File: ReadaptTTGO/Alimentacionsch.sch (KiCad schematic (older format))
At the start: 32 parts, among them J1 USB_B_Micro, J2 Conn_01x02_Shielded, SW1 SW_SPDT, U1 CP2102N-A01-GQFN24, U3 EMH3, U4 TP4054, U5 ME6211, U6 ME6211

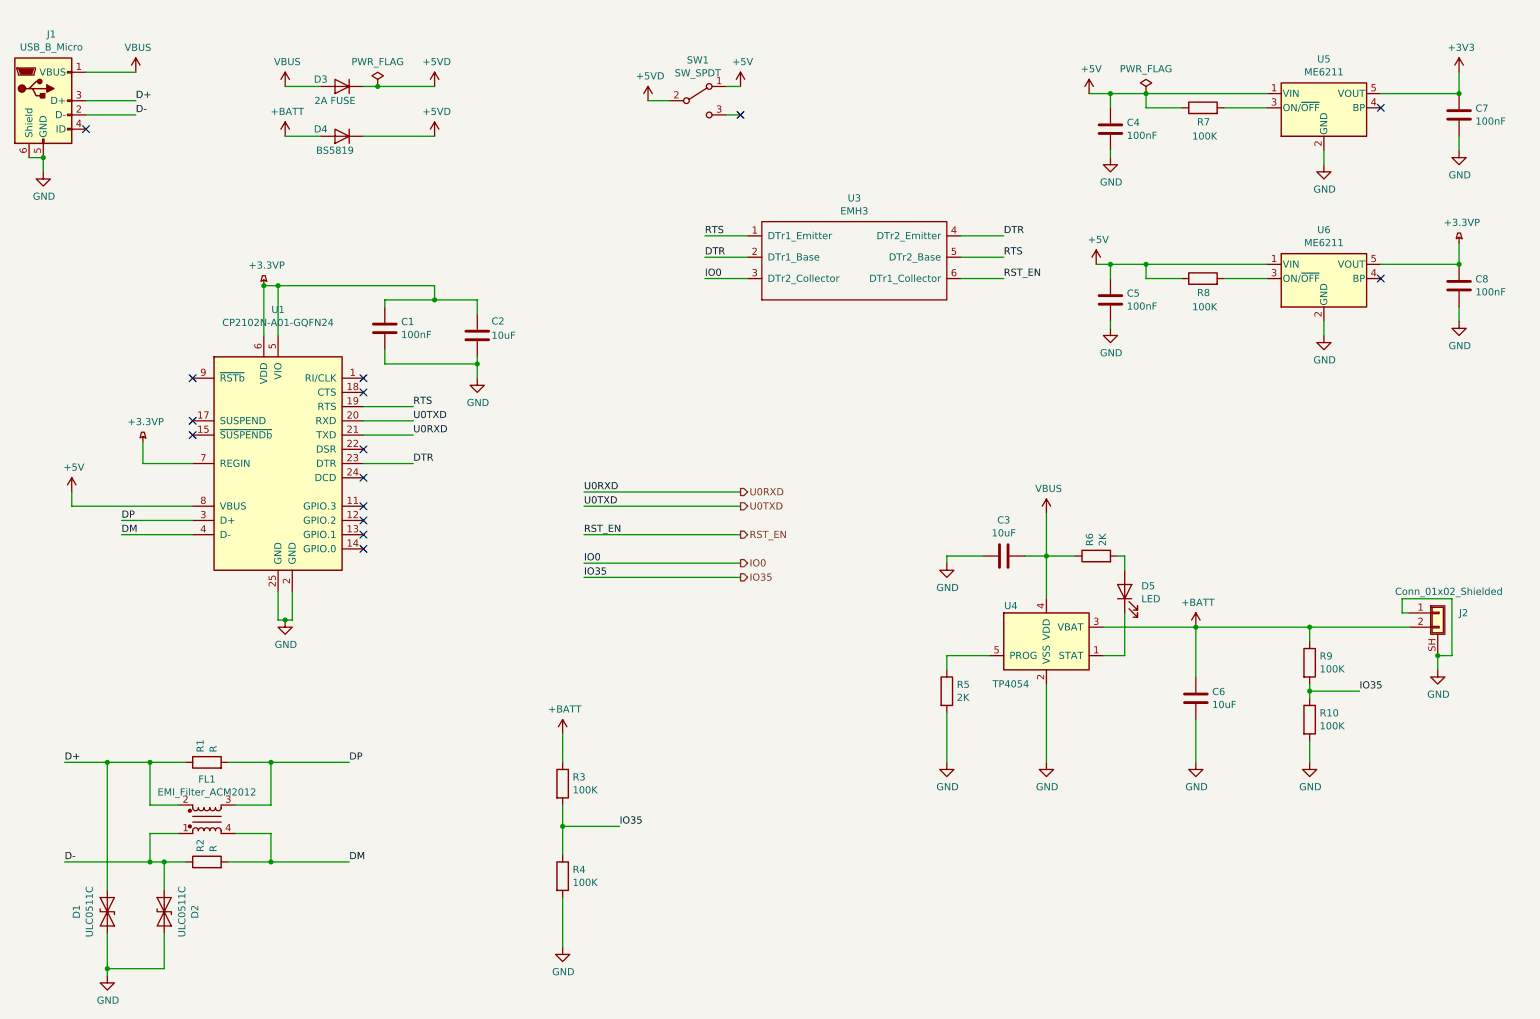
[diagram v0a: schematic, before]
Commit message: Entrega revision 1.2
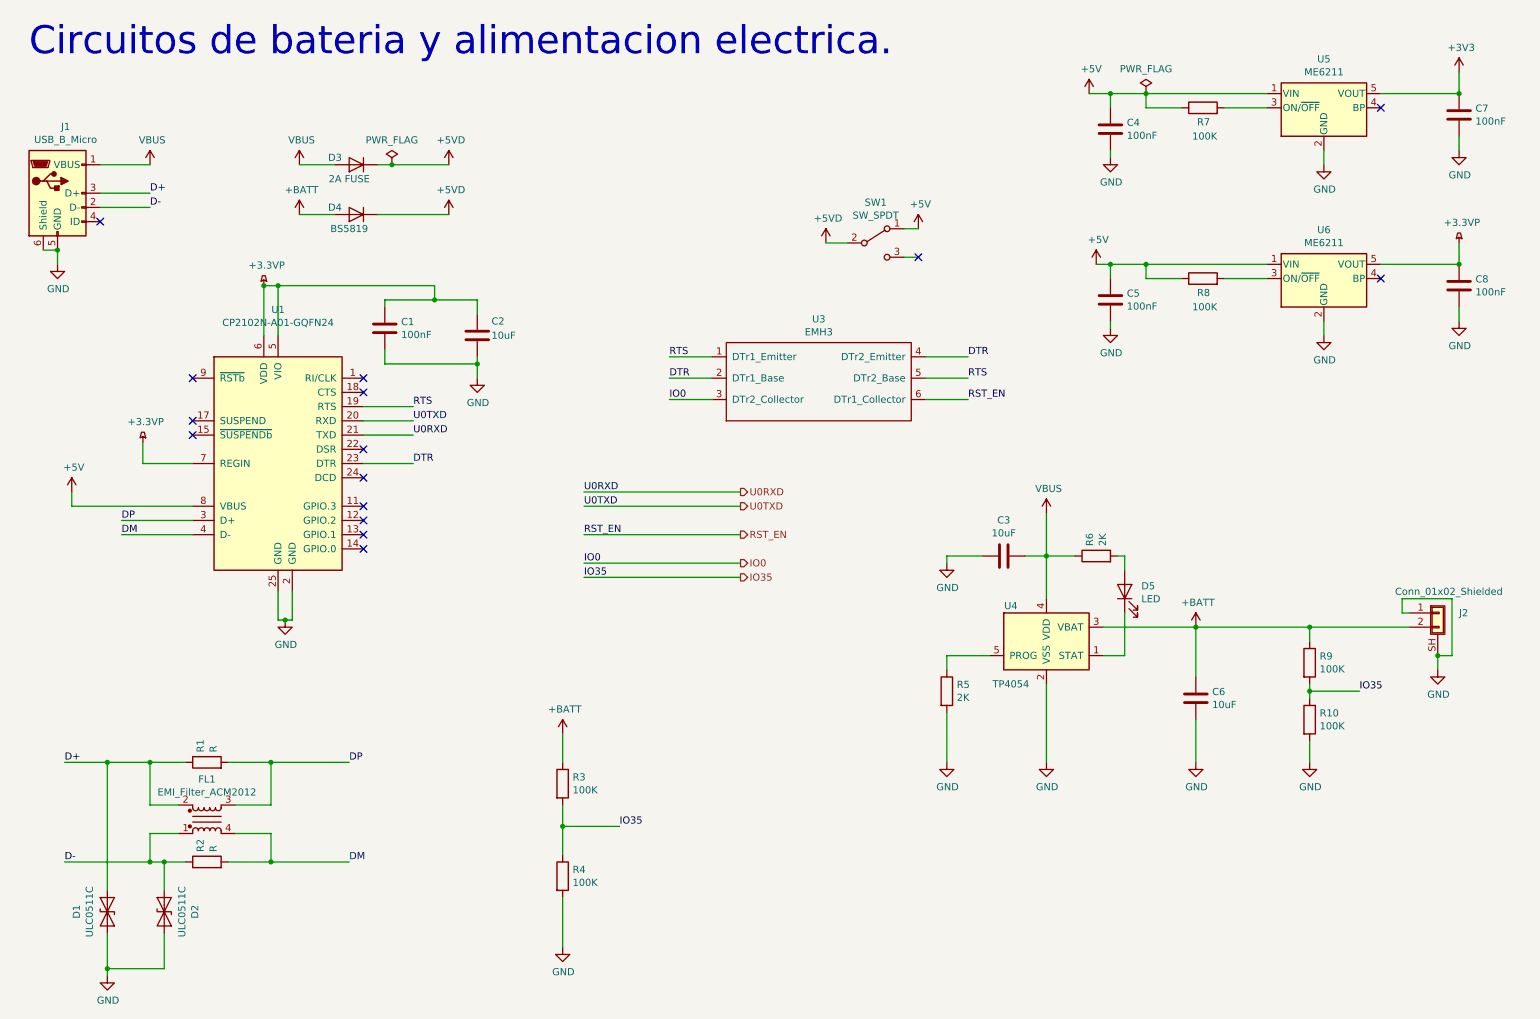
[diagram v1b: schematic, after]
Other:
- note added: "Circuitos de bateria y alimentacion electrica."
- moved on the sheet: D3, D4, J1, SW1, U3
